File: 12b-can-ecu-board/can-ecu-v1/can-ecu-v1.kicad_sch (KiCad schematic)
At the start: 42 parts, among them J1 USB-C, J2 SWD, J3 UART, J4 CAN, SW1 Reset, SW2 Btn1, SW3 Btn2, U1 STM32F407VGTx, U2 AMS1117-3.3, U3 SN65HVD230, U4 LMT86DCK, Y1 8MHz

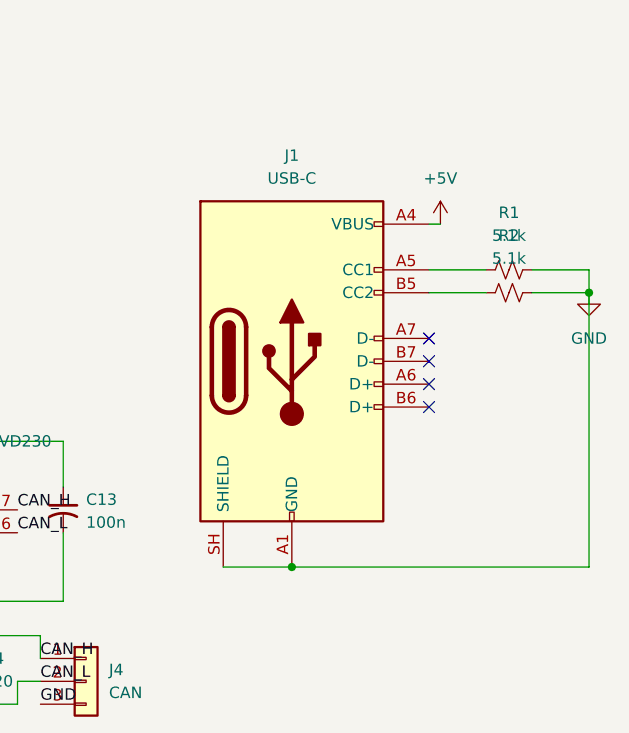
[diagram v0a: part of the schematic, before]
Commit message: 12b-can-ecu-board: first attempt at the schematic. restarting bc errors
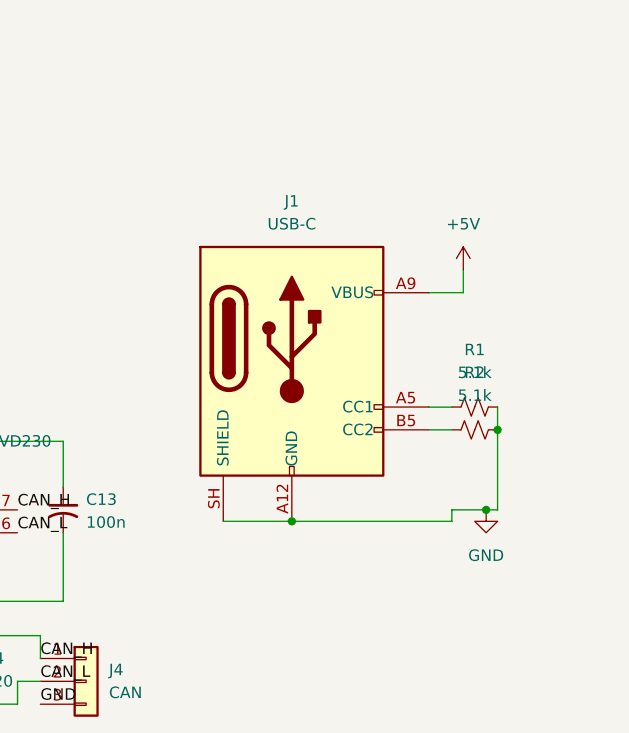
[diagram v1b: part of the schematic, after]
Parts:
- J1: symbol Connector:USB_C_Receptacle_USB2.0_14P -> Connector:USB_C_Receptacle_PowerOnly_6P
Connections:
- net +5V: no longer J1.A4 (VBUS), J1.B4 (VBUS)
- net GND: no longer J1.A1 (GND), J1.B1 (GND)
- no-connect marks 73 -> 69
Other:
- moved on the sheet: R1, R2
